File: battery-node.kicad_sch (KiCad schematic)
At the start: 21 parts, among them J2 Conn_01x02, J3 Conn_01x02, J5 Conn_01x05, J7 TC2050, U1 ESP32-H2-MINI-1-H2S

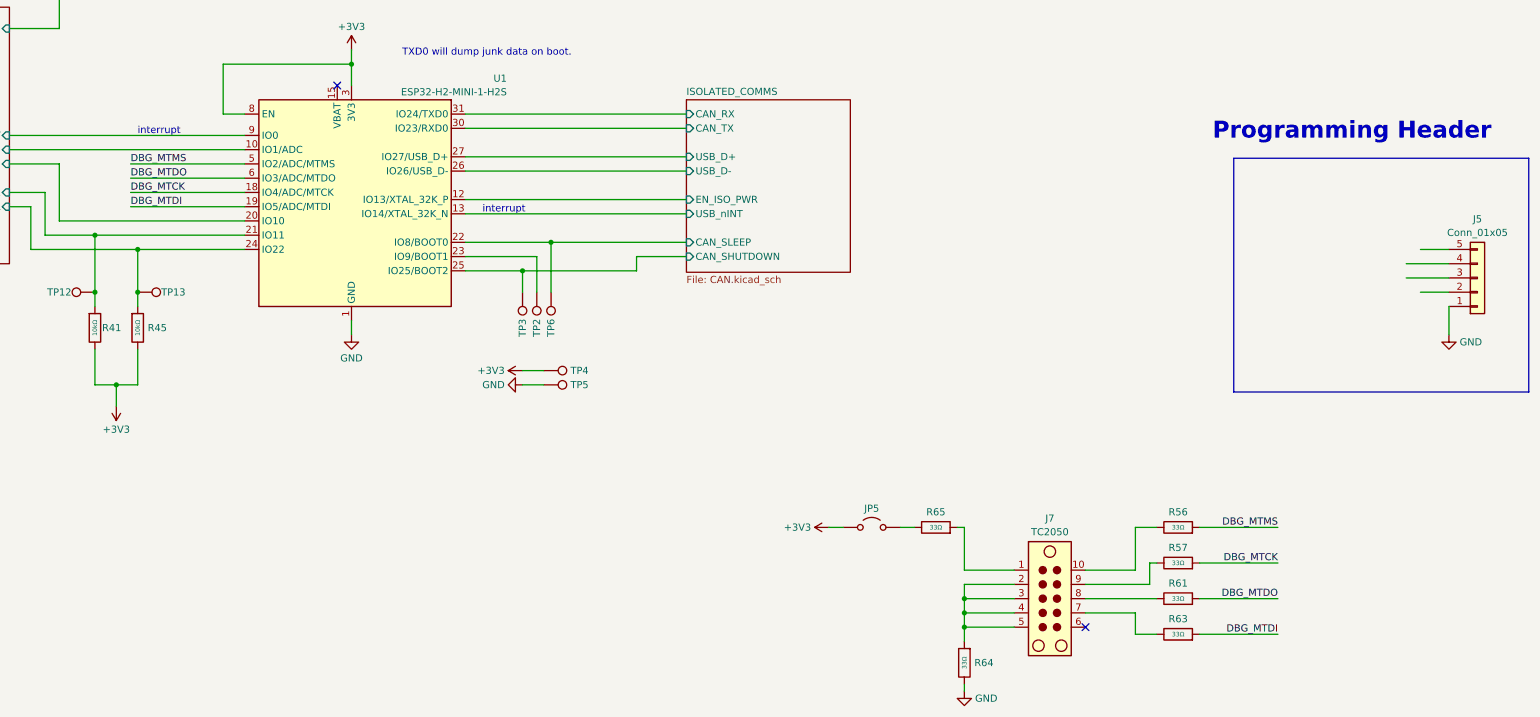
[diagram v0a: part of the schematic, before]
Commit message: rolled back TO commit caa5444, didn't mean to roll THAT back
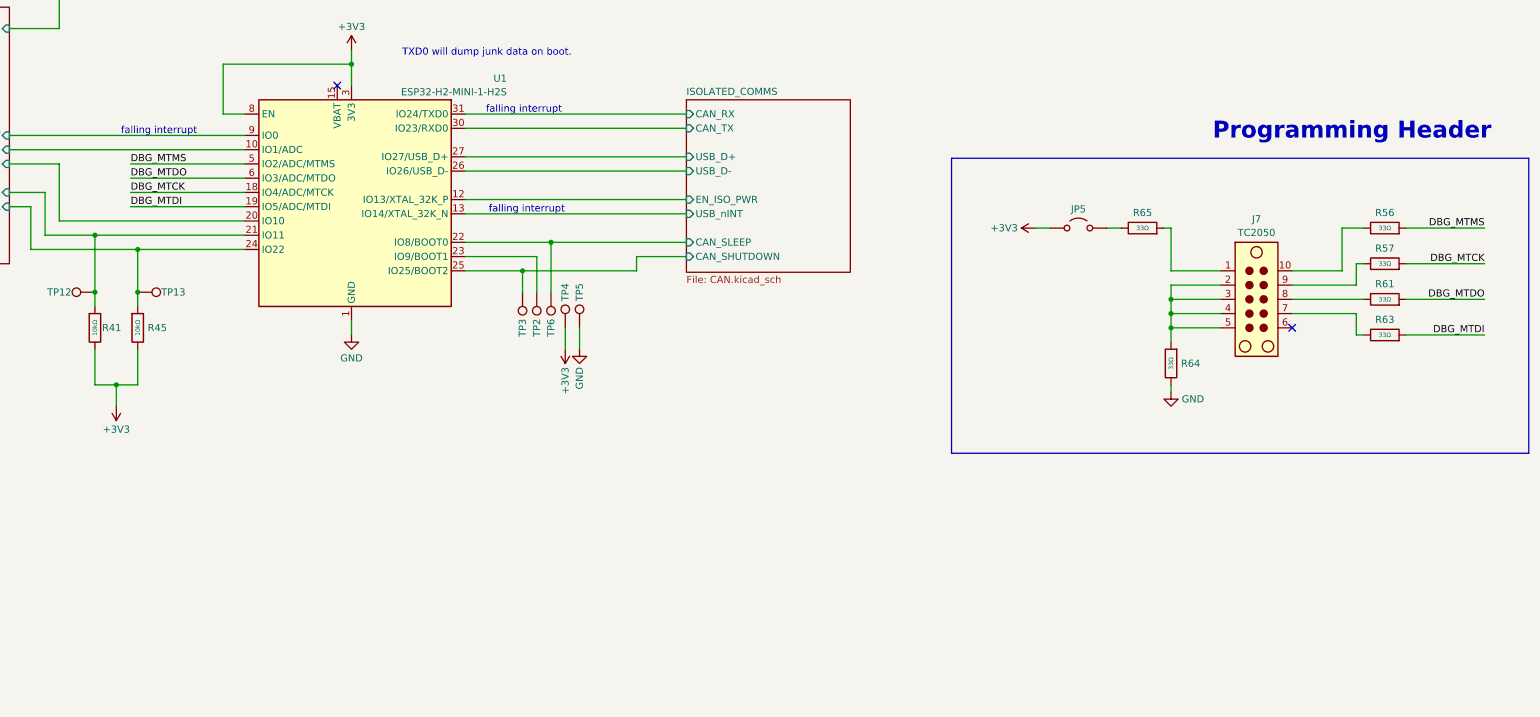
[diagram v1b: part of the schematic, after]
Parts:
- removed J5: Conn_01x05, symbol Connector_Generic:Conn_01x05
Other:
- note added: "falling interrupt"
- note removed: "interrupt"
- moved on the sheet: J7, JP5, R56, R57, R61, R63, R64, R65, TP4, TP5
